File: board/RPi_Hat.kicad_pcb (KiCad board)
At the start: 2 copper layers, 65 x 56 mm, 43 parts, among them J1 PiHat, SW1 Pushbutton, SW2 Pushbutton, SW3 Pushbutton, SW4 Pushbutton, SW5 Pushbutton, SW6 Pushbutton, SW7 Pushbutton, SW8 Pushbutton

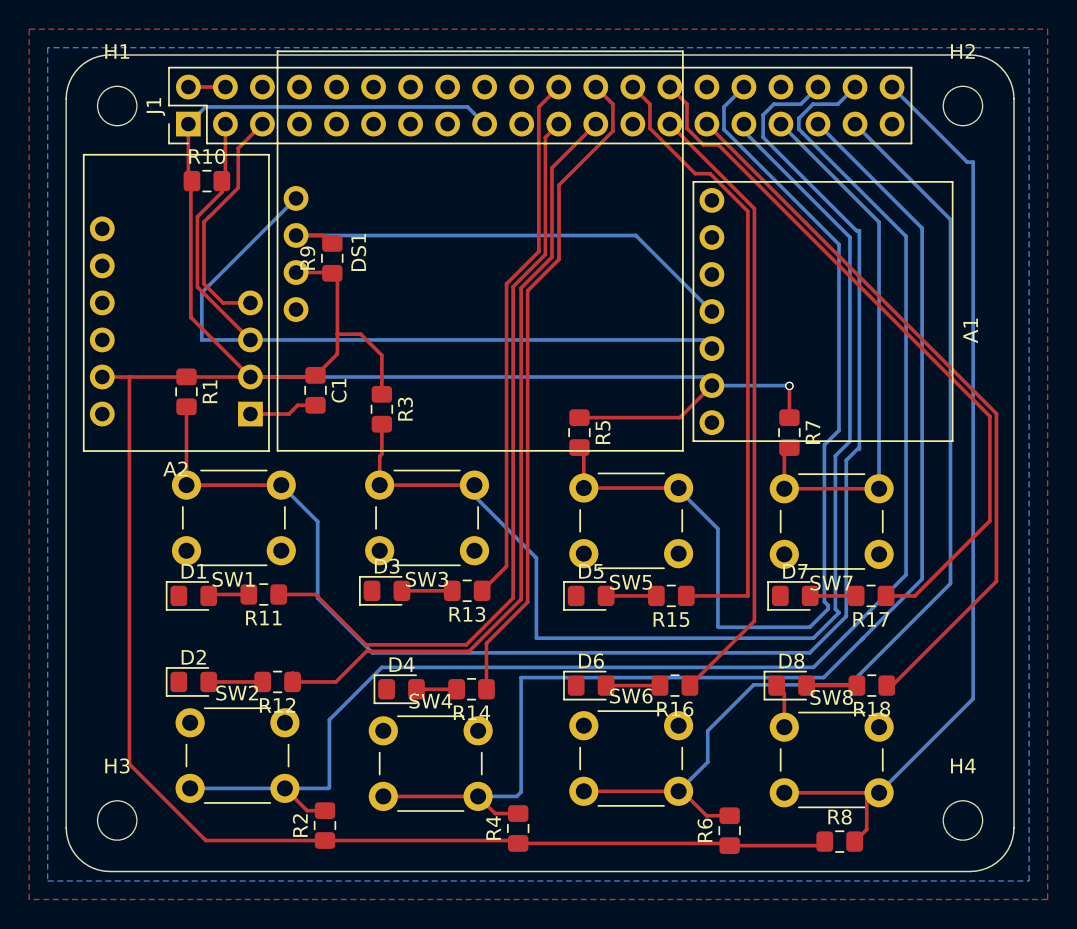
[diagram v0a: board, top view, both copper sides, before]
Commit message: transistors
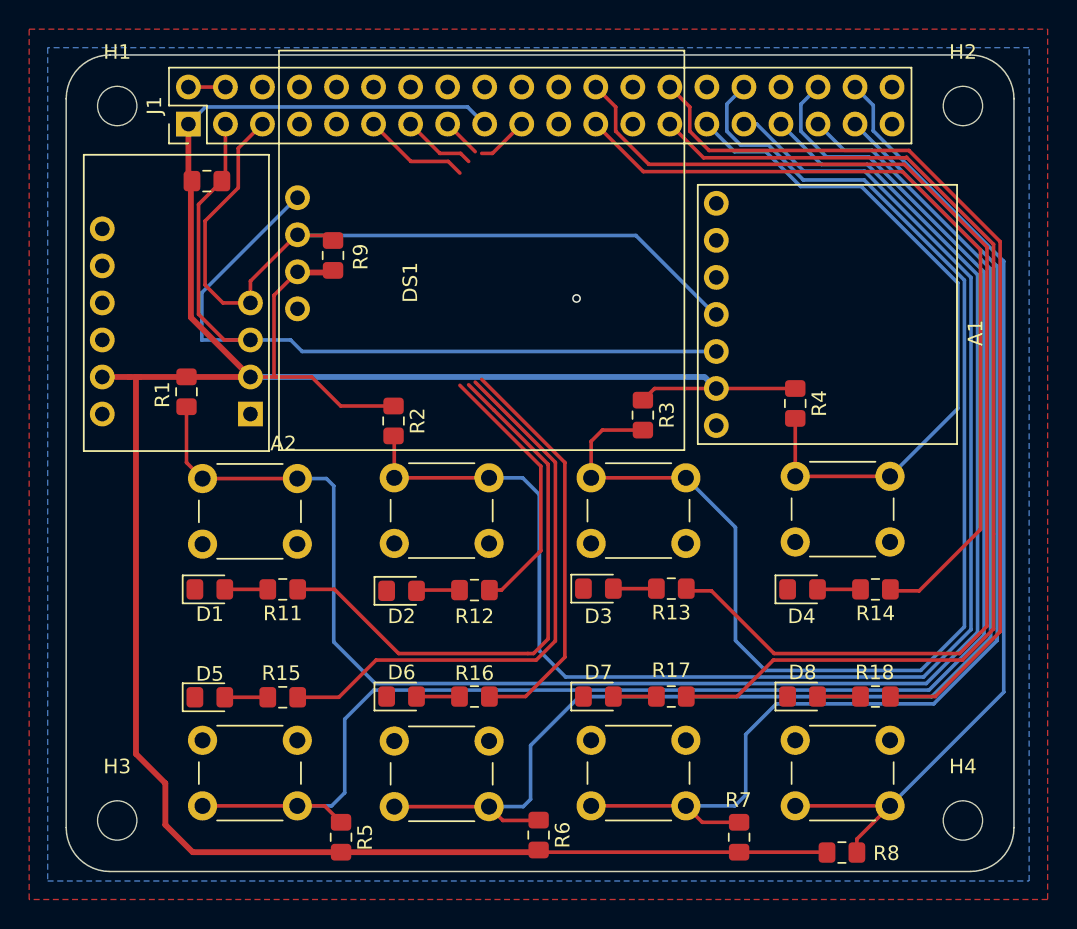
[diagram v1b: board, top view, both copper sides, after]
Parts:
- removed C1: 100n, HWP:C_0805
- moved SW4 37.1 mm to (56.5, 33.9), turned to 180 degrees
- moved SW5 35.1 mm to (9.35, 47.5), turned to 0 degrees
- moved R4 34.8 mm to (50.0, 24.4), turned to -90 degrees
- moved R5 32.2 mm to (18.9, 54.1), turned to 90 degrees
- moved R14 28.5 mm to (55.5, 37.1)
- moved D4 28.3 mm to (50.5, 37.1)
- moved R2 28.1 mm to (22.4, 25.6), turned to -90 degrees
- moved R7 28.0 mm to (46.1, 54.1), turned to 90 degrees
- moved R15 27.5 mm to (14.8, 44.5)
- moved D5 27.1 mm to (9.85, 44.5)
- moved SW2 23.9 mm to (29.0, 34.0), turned to 180 degrees
- moved SW7 23.5 mm to (36.0, 47.5), turned to 0 degrees
- moved R3 17.9 mm to (39.5, 25.2)
- moved D2 15.6 mm to (23.0, 37.2)
- moved R17 15.3 mm to (41.5, 44.5)
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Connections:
- J1 pad 11: unconnected-(J1-Pad11) -> Diode 2
- J1 pad 13: unconnected-(J1-Pad13) -> Diode 1
- J1 pad 15: unconnected-(J1-Pad15) -> Diode 5
- J1 pad 19: unconnected-(J1-Pad19) -> Diode 6
- J1 pad 21: Diode 1 -> unconnected-(J1-Pad21)
- J1 pad 22: Diode 3 -> unconnected-(J1-Pad22)
- J1 pad 23: Diode 2 -> Diode 4
- J1 pad 24: Diode 4 -> Diode 3
- J1 pad 26: Diode 5 -> unconnected-(J1-Pad26)
- J1 pad 27: Diode 6 -> Diode 7
- J1 pad 28: Diode 7 -> Diode 8
- J1 pad 29: Diode 8 -> Button 4
- J1 pad 31: Button 3 -> Button 2
- J1 pad 32: Button 5 -> Button 3
- J1 pad 33: Button 7 -> Button 1
- J1 pad 35: Button 4 -> Button 6
- J1 pad 36: Button 1 -> Button 5
- J1 pad 37: Button 6 -> Button 7
- J1 pad 38: Button 2 -> Button 8
- J1 pad 40: Button 8 -> unconnected-(J1-Pad40)
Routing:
- net Diode 3: track 36.9 -> 81.6 mm
- net Button 5: track 68.3 -> 109.9 mm
- net Button 7: track 37.3 -> 78.5 mm
- net Button 4: track 85.3 -> 47.4 mm
- net Diode 2: track 53.4 -> 25.6 mm
- net Diode 7: track 48.7 -> 75.0 mm
- net Button 6: track 69.8 -> 92.9 mm
- net Diode 8: track 50.1 -> 64.1 mm
- net Button 1: track 101.8 -> 114.4 mm
- net Diode 6: track 42.7 -> 31.3 mm
- net Diode 4: track 45.7 -> 57.1 mm
- net Button 3: track 81.8 -> 91.0 mm
- net GND: track 8.56 -> 0.00 mm, vias 0 -> 1
- net Diode 1: track 52.6 -> 44.1 mm
- net SCL: track 49.8 -> 55.6 mm
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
